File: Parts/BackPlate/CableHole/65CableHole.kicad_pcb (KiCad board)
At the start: 2 copper layers, 172.9 x 20 mm, 3 parts

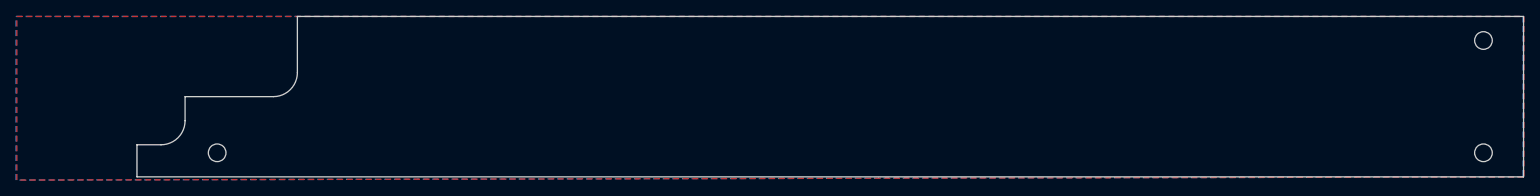
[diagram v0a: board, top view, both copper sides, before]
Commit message: 寸法更新とか
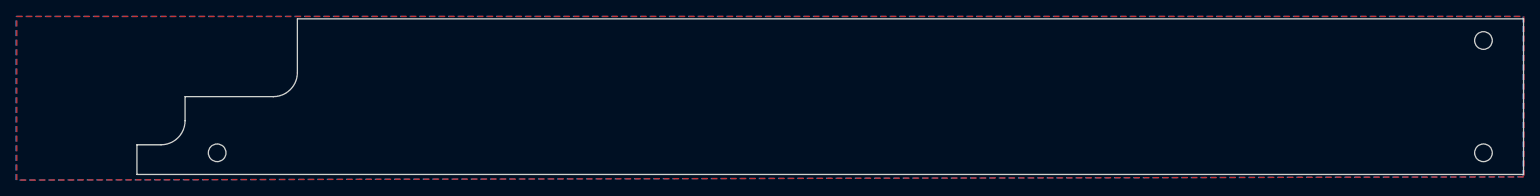
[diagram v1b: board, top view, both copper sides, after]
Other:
- board size 172.9 x 20 mm -> 172.9 x 19.4 mm
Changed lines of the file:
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@@
     (arrow2b (pts (xy 339.75 45.24375) (xy 338.623496 45.830171)))
   )
-  (gr_line (start 186.875 20) (end 339.75 20) (layer Edge.Cuts) (width 0.1))
+  (gr_line (start 186.875 20.3) (end 339.75 20.3) (layer Edge.Cuts) (width 0.1))
   (gr_line (start 172.875 33) (end 172.875 30) (layer Edge.Cuts) (width 0.1))
   (gr_arc (start 169.875 33) (end 169.875 36) (angle -90) (layer Edge.Cuts) (width 0.1))
   (gr_line (start 169.875 36) (end 166.875 36) (layer Edge.Cuts) (width 0.1))
   (gr_arc (start 183.875 27) (end 183.875 30) (angle -90) (layer Edge.Cuts) (width 0.1))
-  (gr_line (start 186.875 27) (end 186.875 20) (layer Edge.Cuts) (width 0.1))
+  (gr_line (start 186.875 27) (end 186.875 20.3) (layer Edge.Cuts) (width 0.1))
   (gr_line (start 172.875 30) (end 183.875 30) (layer Edge.Cuts) (width 0.1))
-  (gr_line (start 166.875 40) (end 166.875 36) (layer Edge.Cuts) (width 0.1))
-  (gr_line (start 339.75 40) (end 339.75 20) (layer Edge.Cuts) (width 0.1))
-  (gr_line (start 166.875 40) (end 339.75 40) (layer Edge.Cuts) (width 0.1))
+  (gr_line (start 166.875 39.7) (end 166.875 36) (layer Edge.Cuts) (width 0.1))
+  (gr_line (start 339.75 39.7) (end 339.75 20.3) (layer Edge.Cuts) (width 0.1))
+  (gr_line (start 166.875 39.7) (end 339.75 39.7) (layer Edge.Cuts) (width 0.1))
   (zone (net 0) (net_name "") (layer F.Cu) (hatch edge 0.508)
     (connect_pads (clearance 0.508))
